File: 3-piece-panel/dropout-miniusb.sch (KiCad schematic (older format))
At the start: 57 parts, among them SW1 Rotary_Encoder_Switch, SW2 SW_Push, U1 ProMicro

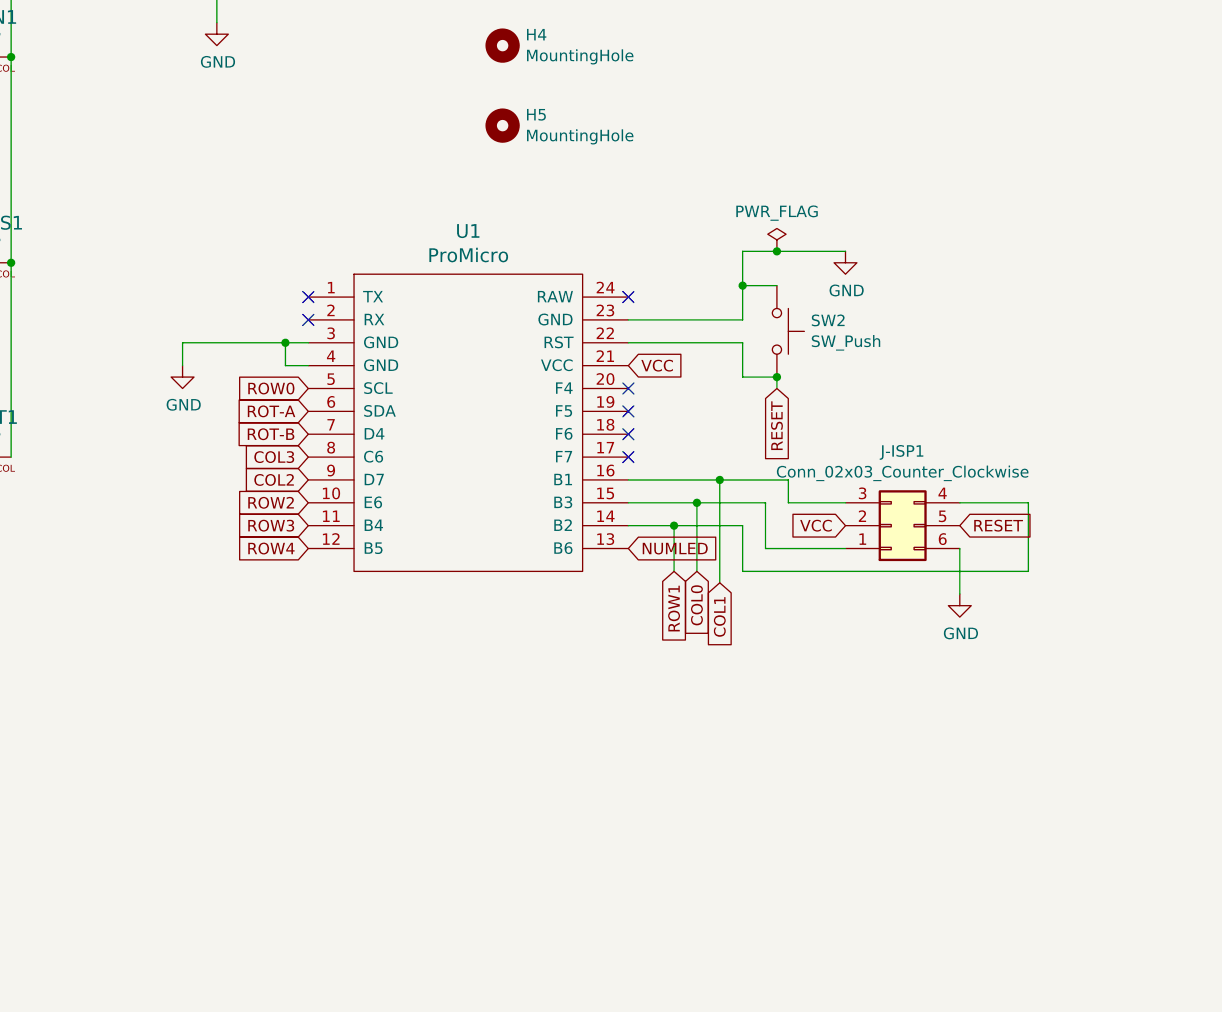
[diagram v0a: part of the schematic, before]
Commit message: rev 0.4
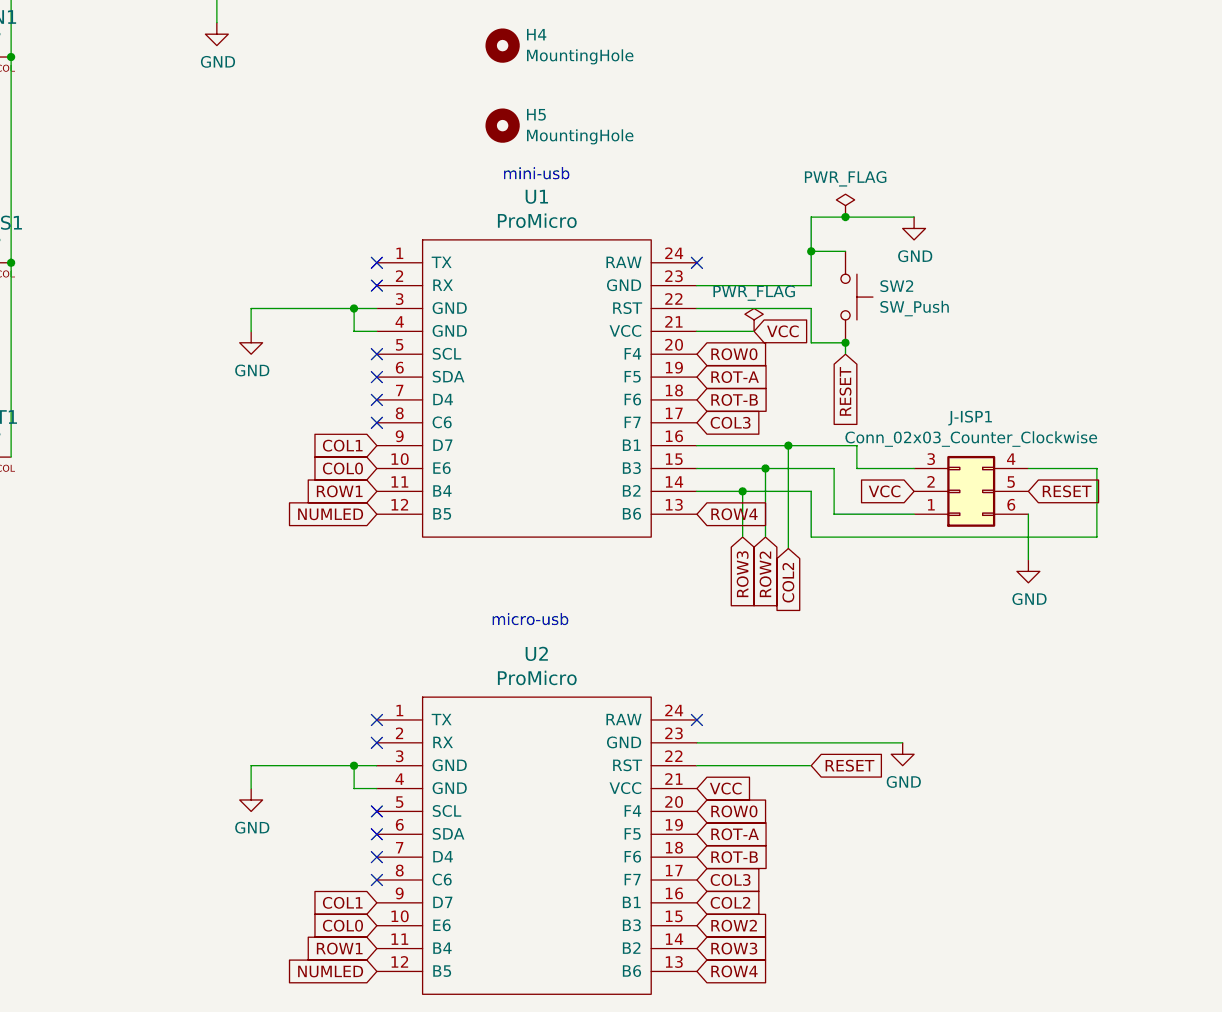
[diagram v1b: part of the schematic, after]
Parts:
- added U2: ProMicro, promicro:ProMicro, symbol promicro:ProMicro
- H10, H11, H12, H13, H14, H15, H6, H7, H8, H9: footprint MountingHole:MountingHole_2.2mm_M2_Pad -> MountingHole:MountingHole_2.2mm_M2
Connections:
- net COL0: now also U1.10 (E6), U2.10 (E6); no longer J-ISP1.1 (Pin_1), U1.15 (B3)
- net COL1: now also U1.9 (D7), U2.9 (D7); no longer J-ISP1.3 (Pin_3), U1.16 (B1)
- net COL2: now also J-ISP1.3 (Pin_3), U1.16 (B1), U2.16 (B1); no longer U1.9 (D7)
- net COL3: now also U1.17 (F7), U2.17 (F7); no longer U1.8 (C6)
- net GND: now also U2.23 (GND), U2.3 (GND), U2.4 (GND)
- net NUMLED: now also U1.12 (B5), U2.12 (B5); no longer U1.13 (B6)
- net RESET: now also U2.22 (RST)
- net ROT-A: now also U1.19 (F5), U2.19 (F5); no longer U1.6 (SDA)
- net ROT-B: now also U1.18 (F6), U2.18 (F6); no longer U1.7 (D4)
- net ROW0: now also U1.20 (F4), U2.20 (F4); no longer U1.5 (SCL)
- net ROW1: now also U1.11 (B4), U2.11 (B4); no longer J-ISP1.4 (Pin_4), U1.14 (B2)
- net ROW2: now also J-ISP1.1 (Pin_1), U1.15 (B3), U2.15 (B3); no longer U1.10 (E6)
- net ROW3: now also J-ISP1.4 (Pin_4), U1.14 (B2), U2.14 (B2); no longer U1.11 (B4)
- net ROW4: now also U1.13 (B6), U2.13 (B6); no longer U1.12 (B5)
- net VCC: now also U2.21 (VCC)
- no-connect marks 7 -> 14
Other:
- note added: "micro-usb\n"
- note added: "mini-usb\n"
- moved on the sheet: J-ISP1, SW2, U1
